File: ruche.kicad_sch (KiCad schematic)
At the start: 32 parts, among them IC2 MAX17048G+, IC3 L86-M33, IC4 SHT41-AD1B-R3, J13 Micro_SD_Card, U1 MKRWAN_1310, U2 MS5611-01BA, U3 XC6220B331MR

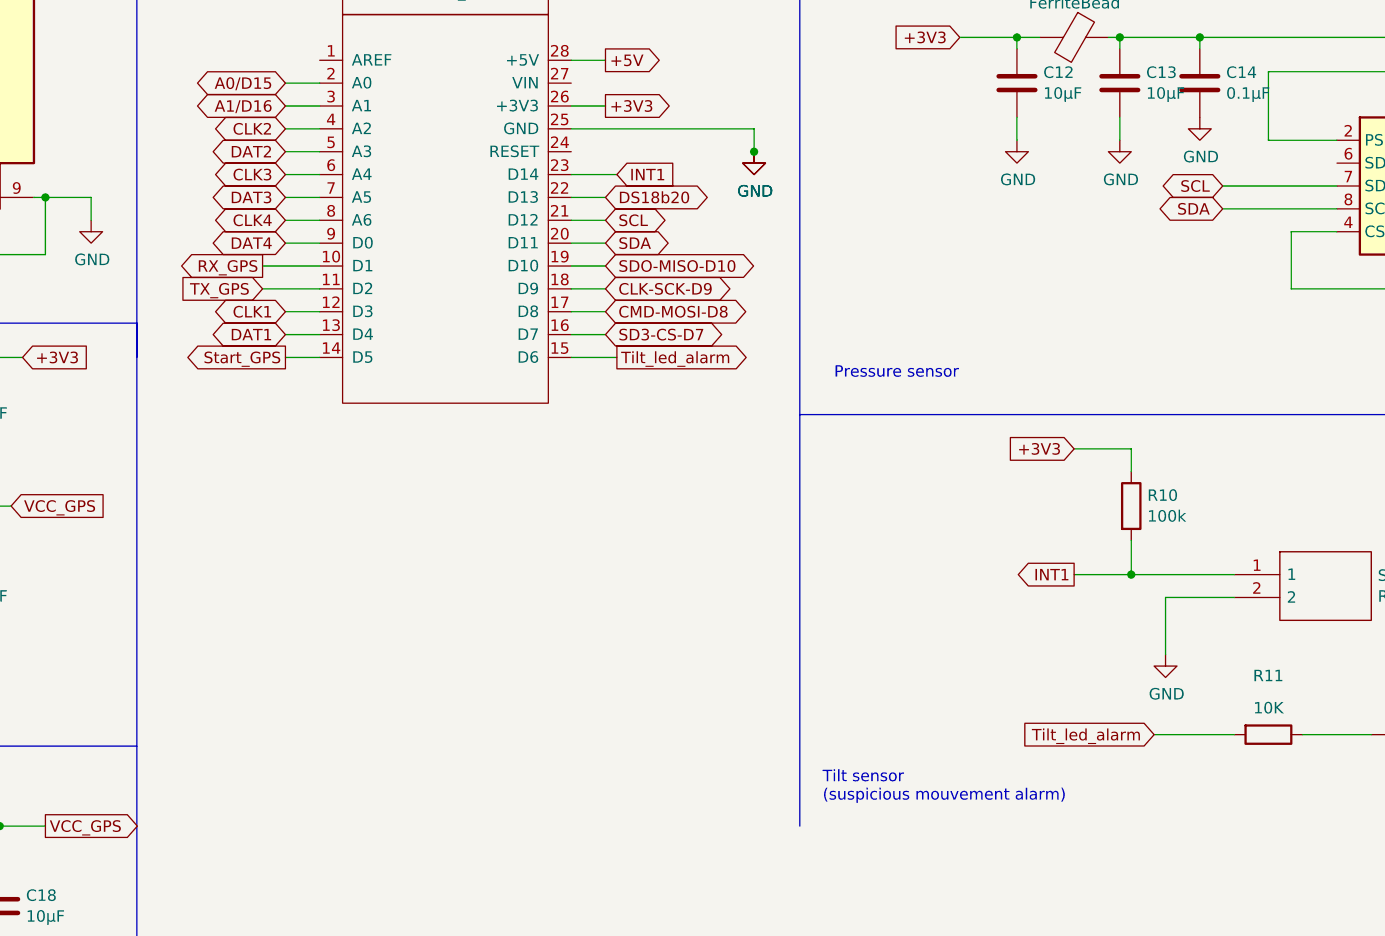
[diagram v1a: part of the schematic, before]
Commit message: V0.2
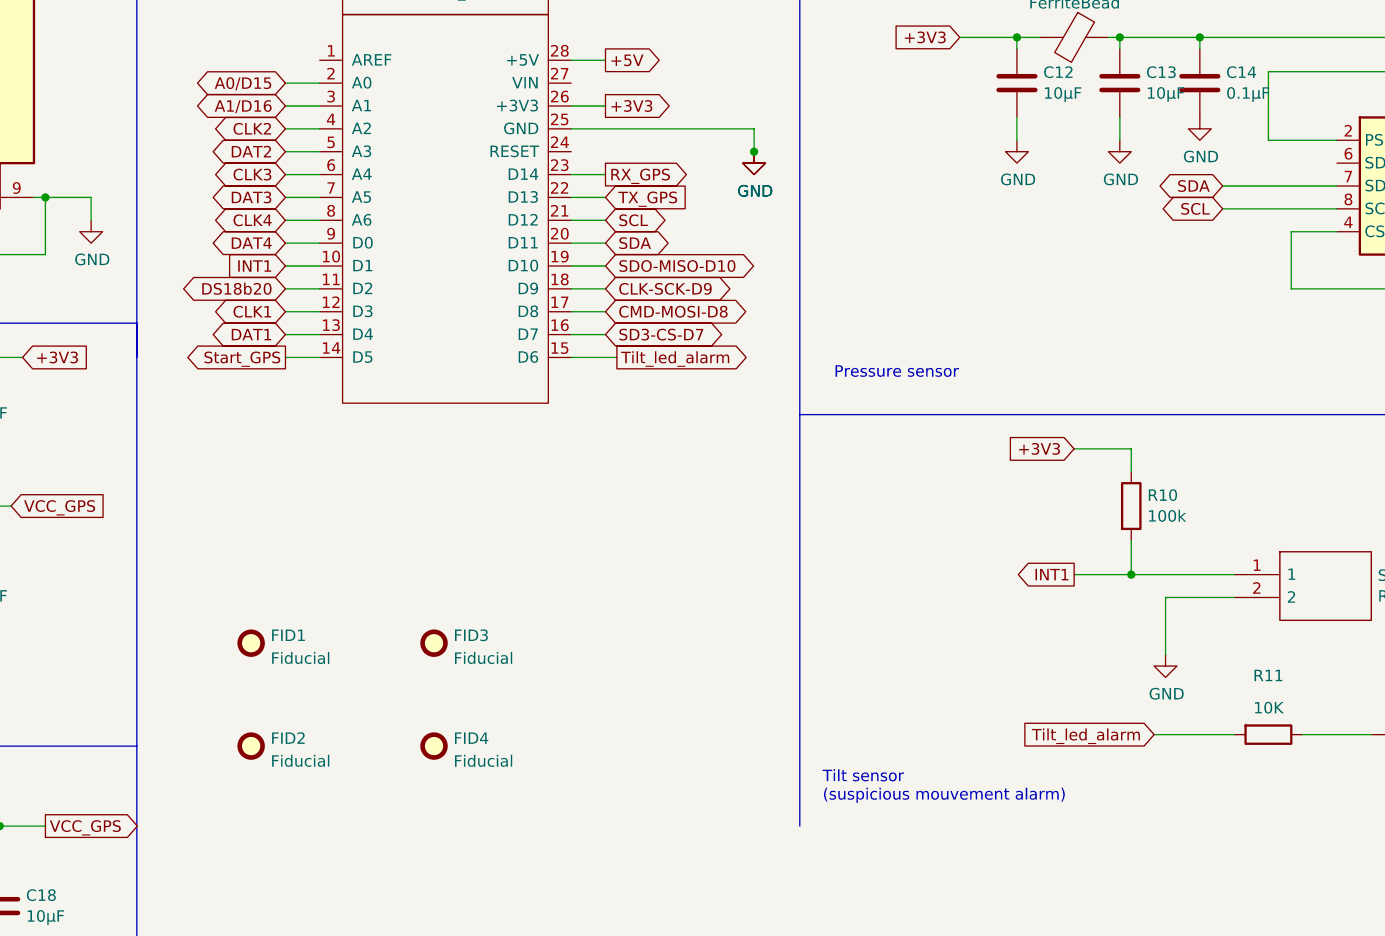
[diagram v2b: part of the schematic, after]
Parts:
- added FID1, FID2, FID3, FID4: Fiducial, Fiducial:Fiducial_1mm_Mask3mm, symbol Mechanical:Fiducial
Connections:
- net DS18b20: now also U1.11 (D2); no longer U1.22 (D13)
- net INT1: now also U1.10 (D1); no longer U1.23 (D14)
- net RX_GPS: now also U1.23 (D14); no longer U1.10 (D1)
- net SCL: now also U2.8 (SCLK); no longer U2.7 (SDI/SDA)
- net SDA: now also U2.7 (SDI/SDA); no longer U2.8 (SCLK)
- net TX_GPS: now also U1.22 (D13); no longer U1.11 (D2)
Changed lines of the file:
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@@
+    (stroke (width 0) (type default) (color 0 0 0 0))
+  )
+  (wire (pts (xy 139.7 106.68) (xy 143.51 106.68))
     (stroke (width 0) (type default) (color 0 0 0 0))
   )
@@
     (stroke (width 0) (type default) (color 0 0 0 0))
   )
+  (wire (pts (xy 171.45 93.98) (xy 175.26 93.98))
+    (stroke (width 0) (type default) (color 0 0 0 0))
+  )
   (wire (pts (xy 237.49 140.97) (xy 237.49 147.32))
     (stroke (width 0) (type default) (color 0 0 0 0))
@@
     (stroke (width 0) (type default) (color 0 0 0 0))
   )
-  (wire (pts (xy 137.16 106.68) (xy 143.51 106.68))
-    (stroke (width 0) (type default) (color 0 0 0 0))
-  )
   (wire (pts (xy 85.09 26.67) (xy 85.09 40.64))
     (stroke (width 0) (type default) (color 0 0 0 0))
@@
     (stroke (width 0) (type default) (color 0 0 0 0))
   )
+  (wire (pts (xy 139.7 104.14) (xy 143.51 104.14))
+    (stroke (width 0) (type default) (color 0 0 0 0))
+  )
   (wire (pts (xy 81.28 179.07) (xy 81.28 181.61))
     (stroke (width 0) (type default) (color 0 0 0 0))
@@
     (stroke (width 0) (type default) (color 0 0 0 0))
   )
-  (wire (pts (xy 175.26 96.52) (xy 171.45 96.52))
-    (stroke (width 0) (type default) (color 0 0 0 0))
-  )
   (wire (pts (xy 252.73 156.21) (xy 260.35 156.21))
     (stroke (width 0) (type default) (color 0 0 0 0))
@@
     (stroke (width 0) (type default) (color 0 0 0 0))
   )
-  (wire (pts (xy 171.45 93.98) (xy 176.53 93.98))
-    (stroke (width 0) (type default) (color 0 0 0 0))
-  )
   (wire (pts (xy 171.45 109.22) (xy 175.26 109.22))
     (stroke (width 0) (type default) (color 0 0 0 0))
@@
     (stroke (width 0) (type default) (color 0 0 0 0))
   )
+  (wire (pts (xy 171.45 96.52) (xy 175.26 96.52))
+    (stroke (width 0) (type default) (color 0 0 0 0))
+  )
   (wire (pts (xy 266.7 85.09) (xy 266.7 82.55))
     (stroke (width 0) (type default) (color 0 0 0 0))
@@
   )
   (wire (pts (xy 53.34 58.42) (xy 53.34 62.23))
-    (stroke (width 0) (type default) (color 0 0 0 0))
-  )
-  (wire (pts (xy 137.16 104.14) (xy 143.51 104.14))
     (stroke (width 0) (type default) (color 0 0 0 0))
   )
@@
     )
   )
-  (global_label "SCL" (shape bidirectional) (at 243.84 95.25 180) (fields_autoplaced)
-    (effects (font (size 1.27 1.27)) (justify right))
-    (property "Intersheet References" "${INTERSHEET_REFS}" (id 0) (at -3.81 -5.08 0)
-      (effects (font (size 1.27 1.27)) hide)
+  (global_label "SDA" (shape bidirectional) (at 243.84 95.25 180) (fields_autoplaced)
+    (effects (font (size 1.27 1.27)) (justify right))
+    (property "Intersheet References" "${INTERSHEET_REFS}" (id 0) (at 237.9477 95.1706 0)
+      (effects (font (size 1.27 1.27)) (justify right) hide)
     )
   )
@@
     )
   )
-  (global_label "DS18b20" (shape bidirectional) (at 175.26 96.52 0) (fields_autoplaced)
-    (effects (font (size 1.27 1.27)) (justify left))
-    (property "Intersheet References" "${INTERSHEET_REFS}" (id 0) (at 113.03 48.26 0)
-      (effects (font (size 1.27 1.27)) hide)
+  (global_label "DS18b20" (shape bidirectional) (at 139.7 106.68 180) (fields_autoplaced)
+    (effects (font (size 1.27 1.27)) (justify right))
+    (property "Intersheet References" "${INTERSHEET_REFS}" (id 0) (at 128.9091 106.6006 0)
+      (effects (font (size 1.27 1.27)) (justify right) hide)
     )
   )
@@
     )
   )
-  (global_label "TX_GPS" (shape input) (at 137.16 106.68 180) (fields_autoplaced)
-    (effects (font (size 1.27 1.27)) (justify right))
-    (property "Intersheet References" "${INTERSHEET_REFS}" (id 0) (at 113.03 48.26 0)
-      (effects (font (size 1.27 1.27)) hide)
+  (global_label "TX_GPS" (shape input) (at 175.26 96.52 0) (fields_autoplaced)
+    (effects (font (size 1.27 1.27)) (justify left))
+    (property "Intersheet References" "${INTERSHEET_REFS}" (id 0) (at 184.4785 96.4406 0)
+      (effects (font (size 1.27 1.27)) (justify left) hide)
     )
   )
@@
     )
   )
-  (global_label "INT1" (shape input) (at 176.53 93.98 0) (fields_autoplaced)
-    (effects (font (size 1.27 1.27)) (justify left))
-    (property "Intersheet References" "${INTERSHEET_REFS}" (id 0) (at 182.9666 93.9006 0)
-      (effects (font (size 1.27 1.27)) (justify left) hide)
+  (global_label "INT1" (shape input) (at 139.7 104.14 180) (fields_autoplaced)
+    (effects (font (size 1.27 1.27)) (justify right))
+    (property "Intersheet References" "${INTERSHEET_REFS}" (id 0) (at 133.2634 104.0606 0)
+      (effects (font (size 1.27 1.27)) (justify right) hide)
     )
   )
@@
     )
   )
-  (global_label "RX_GPS" (shape output) (at 137.16 104.14 180) (fields_autoplaced)
-    (effects (font (size 1.27 1.27)) (justify right))
-    (property "Intersheet References" "${INTERSHEET_REFS}" (id 0) (at 113.03 48.26 0)
-      (effects (font (size 1.27 1.27)) hide)
+  (global_label "RX_GPS" (shape output) (at 175.26 93.98 0) (fields_autoplaced)
+    (effects (font (size 1.27 1.27)) (justify left))
+    (property "Intersheet References" "${INTERSHEET_REFS}" (id 0) (at 184.7809 93.9006 0)
+      (effects (font (size 1.27 1.27)) (justify left) hide)
     )
   )
@@
     )
   )
-  (global_label "SDA" (shape bidirectional) (at 243.84 97.79 180) (fields_autoplaced)
-    (effects (font (size 1.27 1.27)) (justify right))
-    (property "Intersheet References" "${INTERSHEET_REFS}" (id 0) (at -3.81 -5.08 0)
-      (effects (font (size 1.27 1.27)) hide)
+  (global_label "SCL" (shape bidirectional) (at 243.84 97.79 180) (fields_autoplaced)
+    (effects (font (size 1.27 1.27)) (justify right))
+    (property "Intersheet References" "${INTERSHEET_REFS}" (id 0) (at 238.0082 97.7106 0)
+      (effects (font (size 1.27 1.27)) (justify right) hide)
     )
   )
@@
     (pin "2")
   )
+  (symbol (lib_id "Mechanical:Fiducial") (at 135.89 157.48 0) (unit 1)
+    (in_bom yes) (on_board yes) (fields_autoplaced)
+    (property "Reference" "FID2" (id 0) (at 138.049 156.6453 0)
+      (effects (font (size 1.27 1.27)) (justify left))
+    )
+    (property "Value" "Fiducial" (id 1) (at 138.049 159.1822 0)
+      (effects (font (size 1.27 1.27)) (justify left))
+    )
+    (property "Footprint" "Fiducial:Fiducial_1mm_Mask3mm" (id 2) (at 135.89 157.48 0)
+      (effects (font (size 1.27 1.27)) hide)
+    )
+    (property "Datasheet" "~" (id 3) (at 135.89 157.48 0)
+      (effects (font (size 1.27 1.27)) hide)
+    )
+  )
   (symbol (lib_id "Device:C") (at 232.41 83.82 0) (unit 1)
     (in_bom yes) (on_board yes)
@@
     (pin "1")
   )
+  (symbol (lib_id "Mechanical:Fiducial") (at 156.21 146.05 0) (unit 1)
+    (in_bom yes) (on_board yes) (fields_autoplaced)
+    (property "Reference" "FID3" (id 0) (at 158.369 145.2153 0)
+      (effects (font (size 1.27 1.27)) (justify left))
+    )
+    (property "Value" "Fiducial" (id 1) (at 158.369 147.7522 0)
+      (effects (font (size 1.27 1.27)) (justify left))
+    )
+    (property "Footprint" "Fiducial:Fiducial_1mm_Mask3mm" (id 2) (at 156.21 146.05 0)
+      (effects (font (size 1.27 1.27)) hide)
+    )
+    (property "Datasheet" "~" (id 3) (at 156.21 146.05 0)
+      (effects (font (size 1.27 1.27)) hide)
+    )
+  )
   (symbol (lib_id "Device:R") (at 44.45 66.04 0) (unit 1)
     (in_bom yes) (on_board yes)
@@
     (pin "1")
   )
+  (symbol (lib_id "Mechanical:Fiducial") (at 135.89 146.05 0) (unit 1)
+    (in_bom yes) (on_board yes) (fields_autoplaced)
+    (property "Reference" "FID1" (id 0) (at 138.049 145.2153 0)
+      (effects (font (size 1.27 1.27)) (justify left))
+    )
+    (property "Value" "Fiducial" (id 1) (at 138.049 147.7522 0)
+      (effects (font (size 1.27 1.27)) (justify left))
+    )
+    (property "Footprint" "Fiducial:Fiducial_1mm_Mask3mm" (id 2) (at 135.89 146.05 0)
+      (effects (font (size 1.27 1.27)) hide)
+    )
+    (property "Datasheet" "~" (id 3) (at 135.89 146.05 0)
+      (effects (font (size 1.27 1.27)) hide)
+    )
+  )
   (symbol (lib_id "power:GND") (at 266.7 110.49 0) (unit 1)
     (in_bom yes) (on_board yes)
@@
     )
     (pin "1")
+  )
+  (symbol (lib_id "Mechanical:Fiducial") (at 156.21 157.48 0) (unit 1)
+    (in_bom yes) (on_board yes) (fields_autoplaced)
+    (property "Reference" "FID4" (id 0) (at 158.369 156.6453 0)
+      (effects (font (size 1.27 1.27)) (justify left))
+    )
+    (property "Value" "Fiducial" (id 1) (at 158.369 159.1822 0)
+      (effects (font (size 1.27 1.27)) (justify left))
+    )
+    (property "Footprint" "Fiducial:Fiducial_1mm_Mask3mm" (id 2) (at 156.21 157.48 0)
+      (effects (font (size 1.27 1.27)) hide)
+    )
+    (property "Datasheet" "~" (id 3) (at 156.21 157.48 0)
+      (effects (font (size 1.27 1.27)) hide)
+    )
   )
   (symbol (lib_id "power:GND") (at 118.11 99.06 0) (unit 1)
@@
       (reference "FB1") (unit 1) (value "FerriteBead") (footprint "Resistor_SMD:R_0603_1608Metric")
     )
+    (path "/86bdc510-c778-45e0-b037-11148ebcd2d4"
+      (reference "FID1") (unit 1) (value "Fiducial") (footprint "Fiducial:Fiducial_1mm_Mask3mm")
+    )
+    (path "/2c608864-e6af-45e6-811b-5efe3309d320"
+      (reference "FID2") (unit 1) (value "Fiducial") (footprint "Fiducial:Fiducial_1mm_Mask3mm")
+    )
+    (path "/7982a1f2-441d-4ddf-b0ba-97db71059f0f"
+      (reference "FID3") (unit 1) (value "Fiducial") (footprint "Fiducial:Fiducial_1mm_Mask3mm")
+    )
+    (path "/965affb2-c3f4-484e-9c0a-0b5682f1b69d"
+      (reference "FID4") (unit 1) (value "Fiducial") (footprint "Fiducial:Fiducial_1mm_Mask3mm")
+    )
     (path "/00000000-0000-0000-0000-0000609e7af1/31c6505b-fdd9-40cc-a280-26c0fa241def"
